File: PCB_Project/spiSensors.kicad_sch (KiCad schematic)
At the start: 10 parts

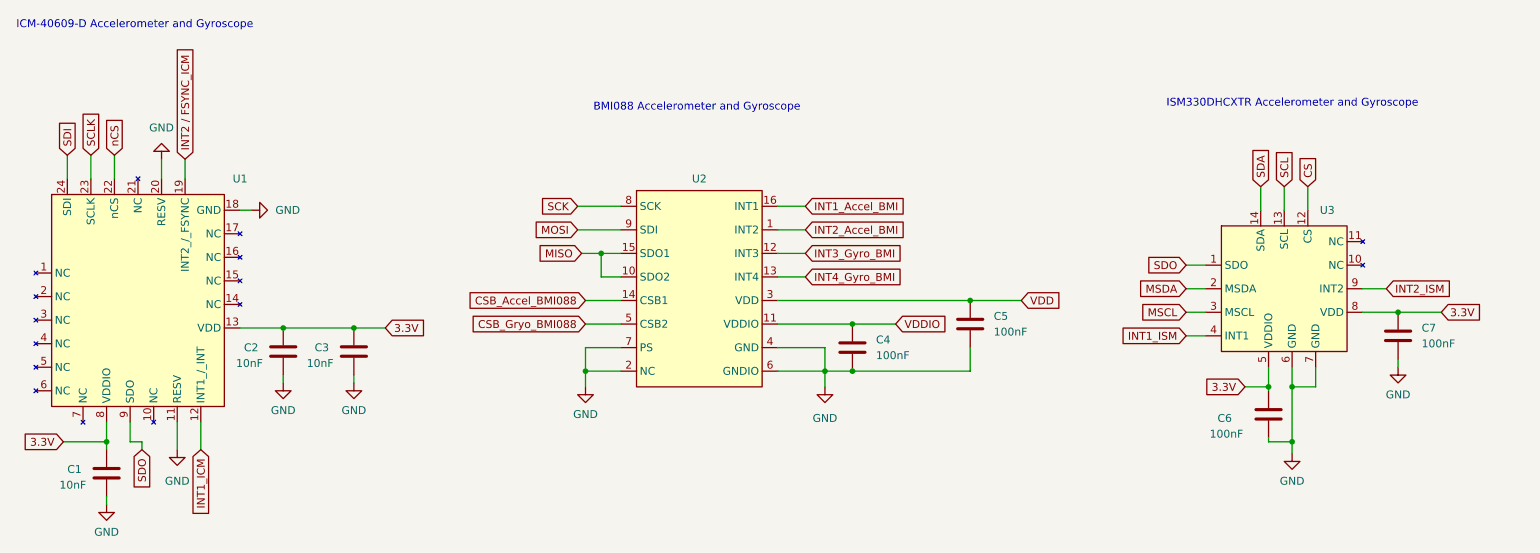
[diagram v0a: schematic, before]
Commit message: cleanup
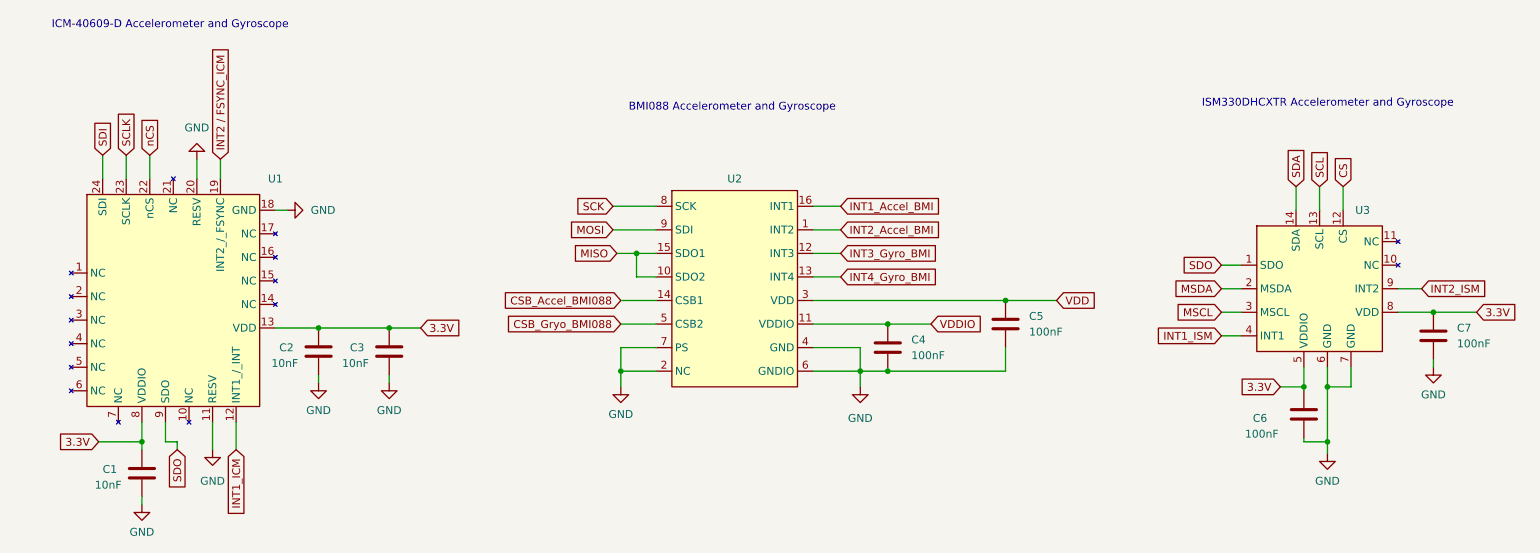
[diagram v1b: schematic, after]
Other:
- moved on the sheet: C1, C2, C3, C4, C5, C6, C7, U1, U2, U3
